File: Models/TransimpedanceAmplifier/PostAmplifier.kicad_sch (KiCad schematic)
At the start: 16 parts, among them Q1 Q_PNP, Q2 Q_NPN, U6 OP37GSZ

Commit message: Finished for today
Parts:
- C19, C20: Purchase Link (none) -> https://www.digikey.com/en/products/detail/murata-electroni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
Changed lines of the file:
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@@
 			)
 		)
-		(property "Purchase Link" ""
+		(property "Purchase Link" "https://www.digikey.com/en/products/detail/murata-electronics/GRM188R72A104KA35D/702549"
 			(at 137.16 54.61 0)
 			(effects
@@
 			)
 		)
-		(property "Purchase Link" ""
+		(property "Purchase Link" "https://www.digikey.com/en/products/detail/murata-electronics/GRM188R72A104KA35D/702549"
 			(at 55.88 77.47 0)
 			(effects

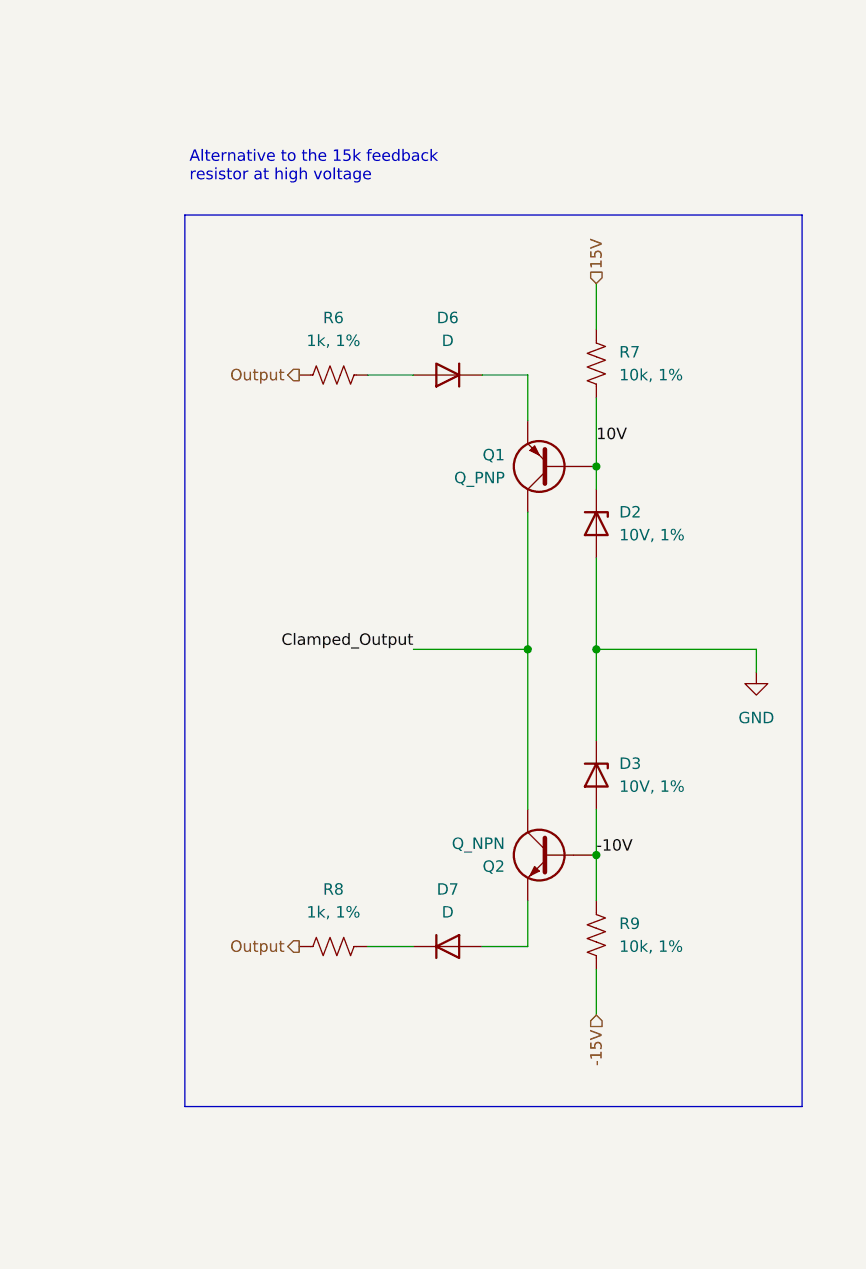
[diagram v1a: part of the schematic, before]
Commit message: Save progress
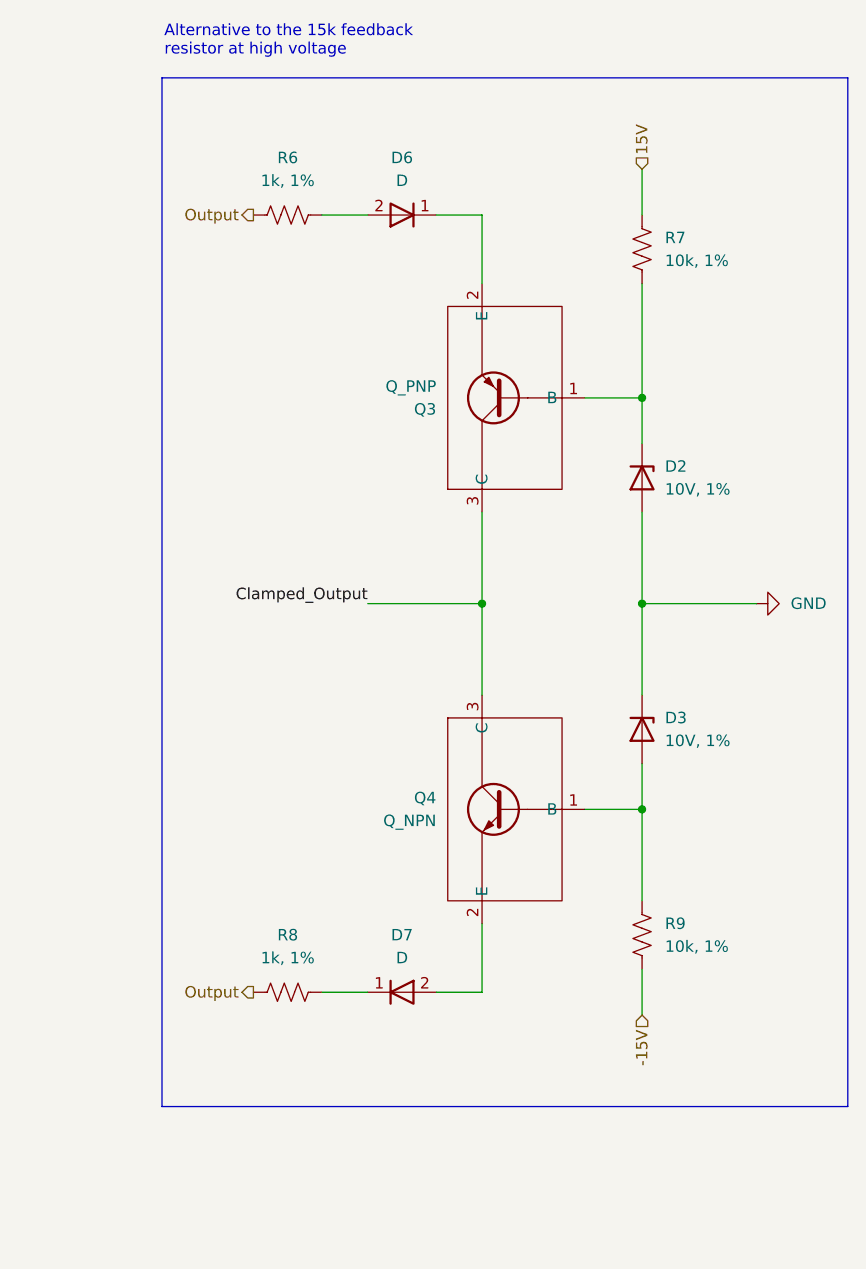
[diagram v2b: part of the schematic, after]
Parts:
- removed Q1: Q_PNP, symbol Device:Q_PNP
- removed Q2: Q_NPN, symbol Device:Q_NPN
- added Q3: Q_PNP, symbol Custom:Q_PNP
- added Q4: Q_NPN, symbol Custom:Q_NPN
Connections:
- net Clamped_Output: now also Q3.3 (C), Q4.3 (C)
- net at D6.1 (K): now also Q3.2 (E)
- net at D7.2 (A): now also Q4.2 (E)
- net -10V: no longer names the net of D3.2 (A), R9.1
- net -10V: now also Q4.1 (B)
- net 10V: no longer names the net of D2.1 (K), R7.2
- net 10V: now also Q3.1 (B)
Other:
- moved on the sheet: D2, D3, R6, R7, R8, R9

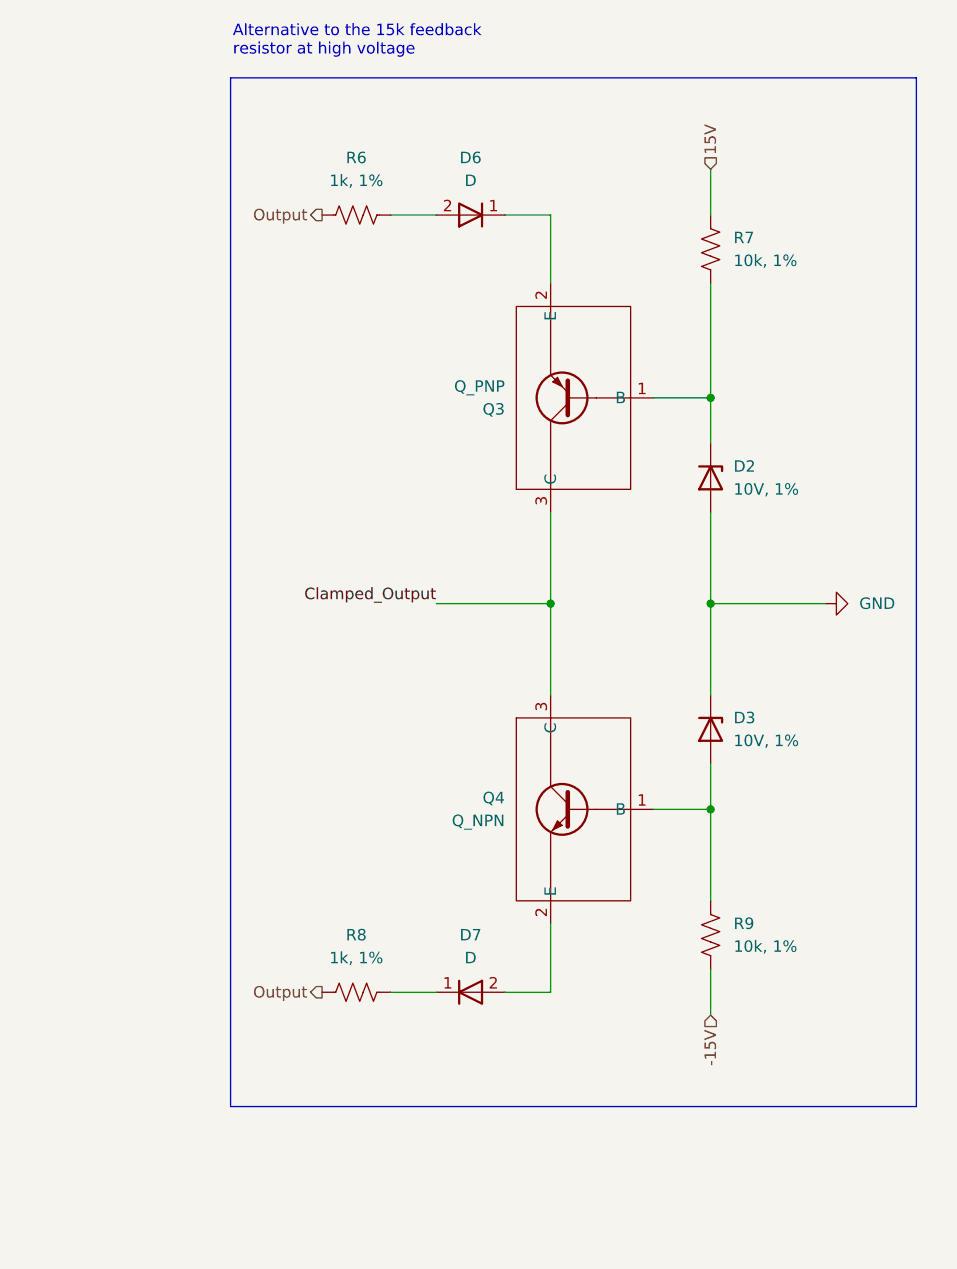
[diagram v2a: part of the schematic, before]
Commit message: Save progress
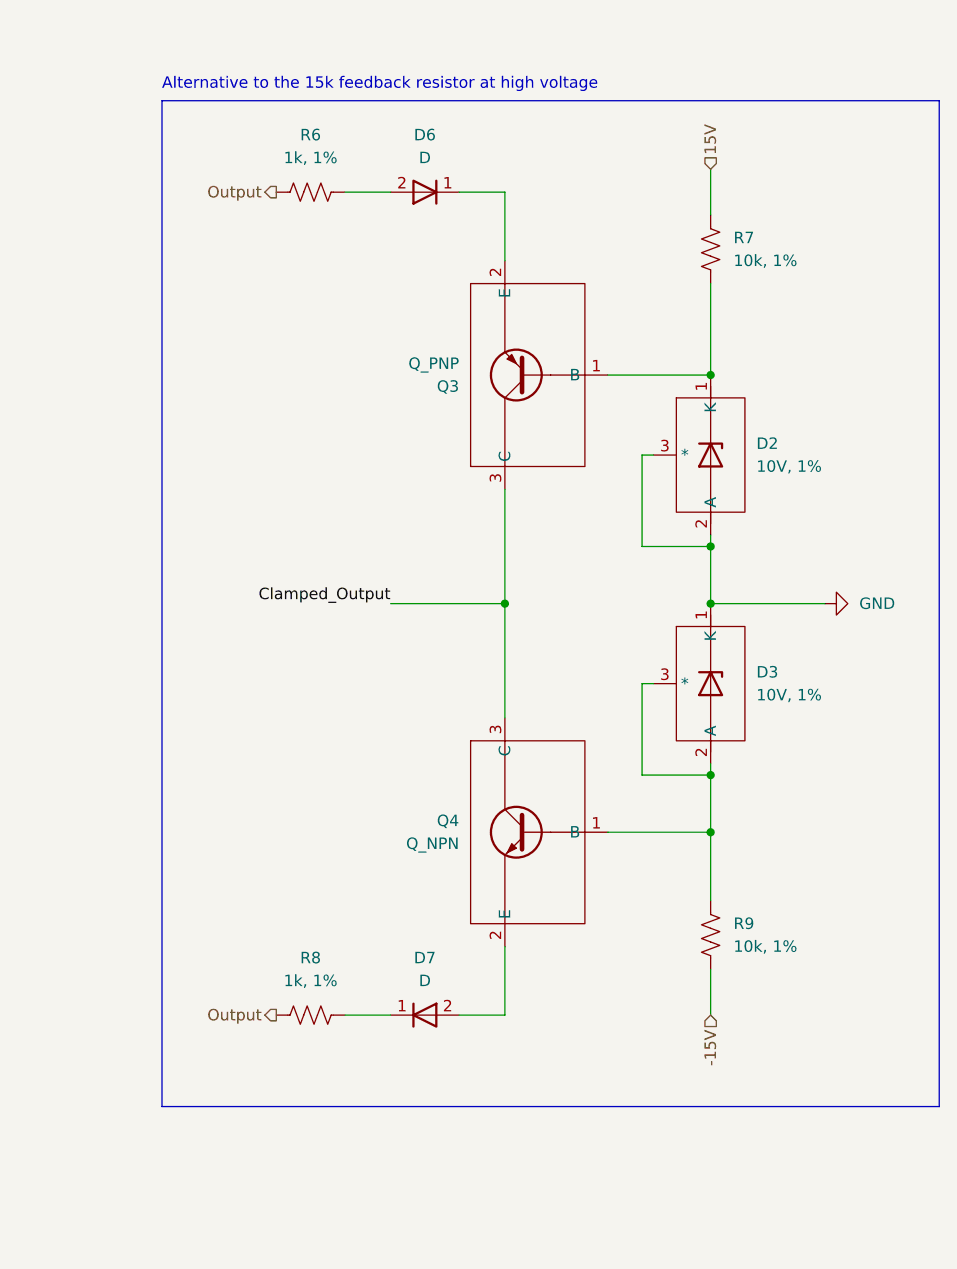
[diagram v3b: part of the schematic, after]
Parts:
- removed D2, D3: 10V, 1%, symbol Device:D_Zener
- added D2, D3: 10V, 1%, symbol Custom:D_Zener
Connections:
- net GND: now also D2.2 (A), D2.3 (*), D3.1 (K)
- net at Q3.1 (B), R7.2: now also D2.1 (K)
- net at Q4.1 (B), R9.1: now also D3.2 (A), D3.3 (*)
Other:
- moved on the sheet: D6, D7, Q3, Q4, R6, R8
